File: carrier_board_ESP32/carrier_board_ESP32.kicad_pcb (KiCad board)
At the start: 4 copper layers, 100 x 100 mm, 49 parts, among them J1 Conn_01x02_Socket, J12 LTR390, J13 BME280, J14 ENS160 SPI, J15 ENS160 + AHT21, J16 ENS160 I2C, J17 Conn_01x22_Socket, J18 Conn_01x22_Socket, J2 Conn_01x02_Socket, J3 UJC-HP-3-SMT-TR, U1 TP4056, U2 LM2576HVS-5, U3 MT3608, U4 ESP32-S3-DEVKITC-1-N8R2

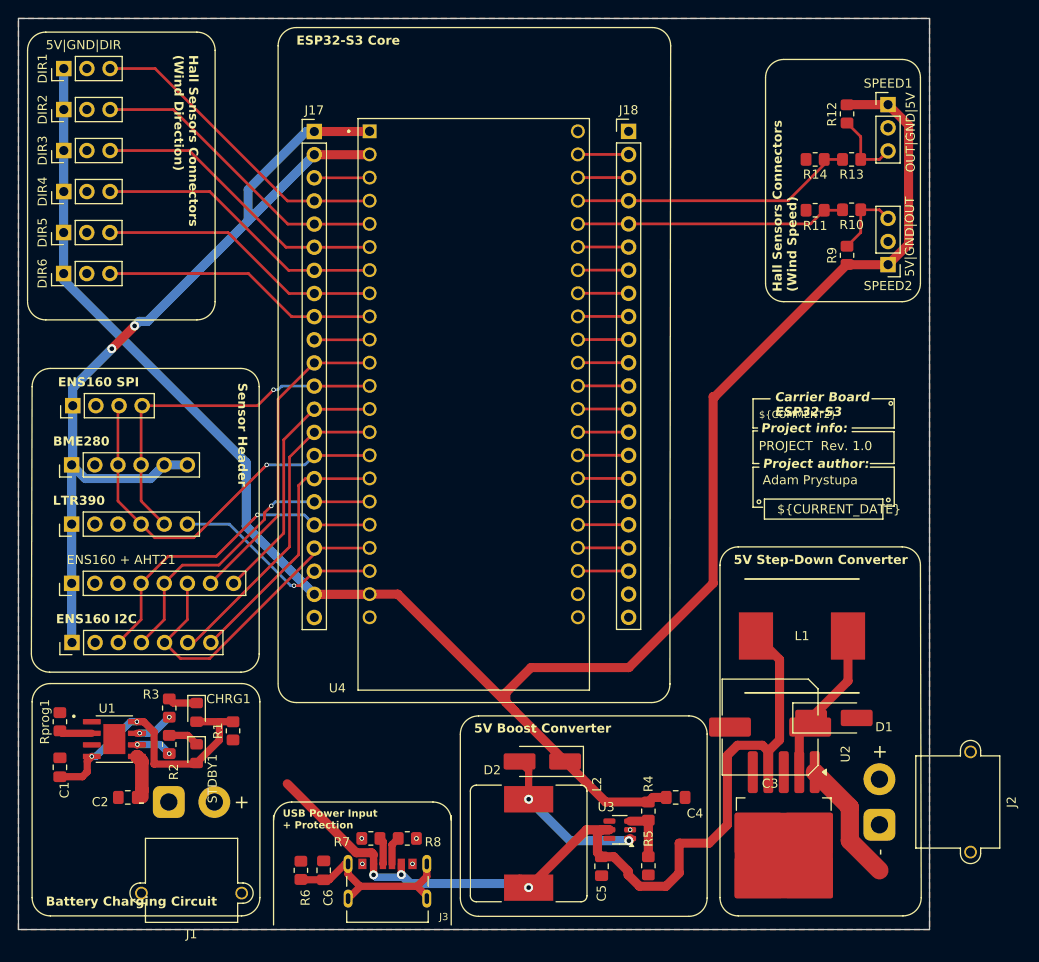
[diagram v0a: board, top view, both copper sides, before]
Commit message: updated scheme and PCB ready for inspection
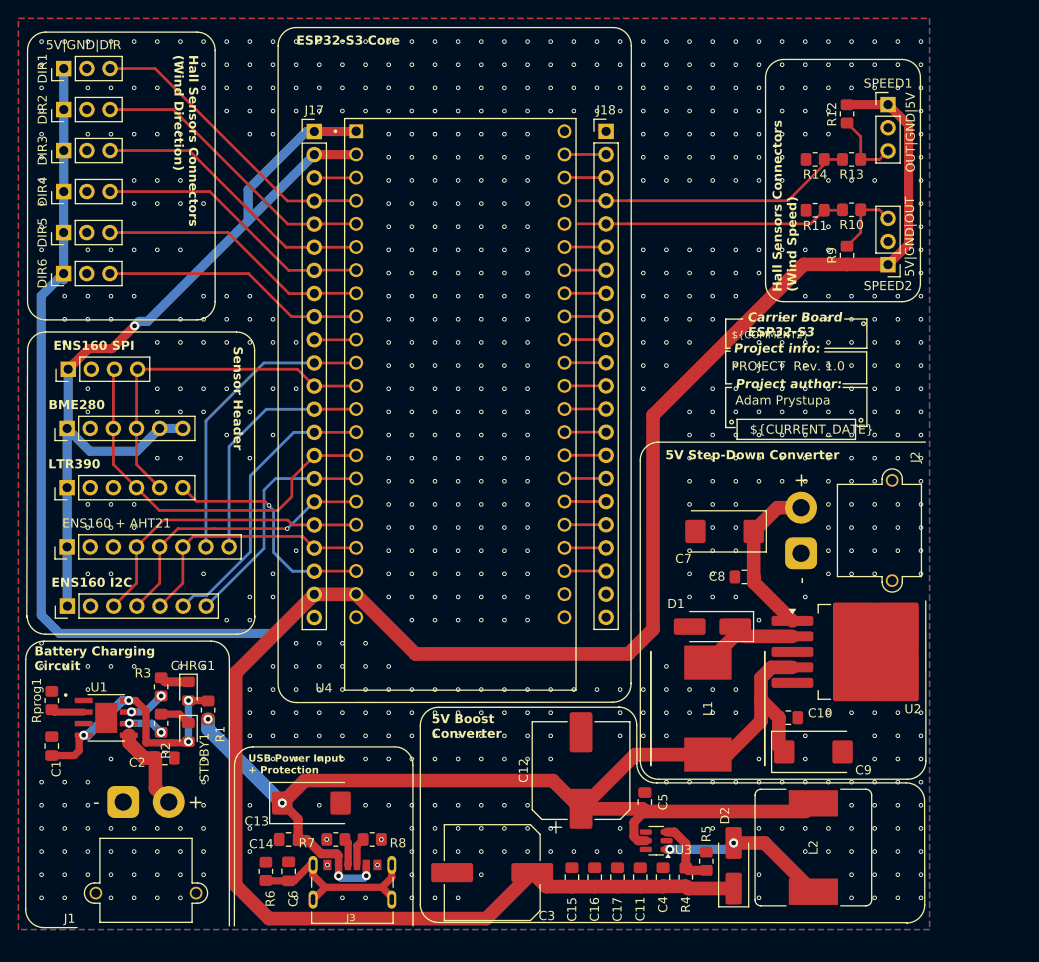
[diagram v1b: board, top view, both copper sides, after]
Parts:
- added C10: 10uF, Capacitor_SMD:C_0805_2012Metric_Pad1.18x1.45mm_HandSolder, F.Cu at (263.0, 98.2)
- added C11: 47uF, Capacitor_SMD:C_0805_2012Metric_Pad1.18x1.45mm_HandSolder, F.Cu at (246.8, 115.8)
- added C12: 2200uF, Capacitor_SMD:CP_Elec_10x10.5, F.Cu at (240.2, 104.0)
- added C13: 10uF, Capacitor_Tantalum_SMD:CP_EIA-7343-15_Kemet-W_Pad2.25x2.55mm_HandSolder, F.Cu at (210.7, 107.6)
- added C14: 1uF, Capacitor_SMD:C_0805_2012Metric_Pad1.18x1.45mm_HandSolder, F.Cu at (208.2, 111.6)
- added C15: 10uF, Capacitor_SMD:C_0805_2012Metric_Pad1.18x1.45mm_HandSolder, F.Cu at (239.2, 115.8)
- added C16: 10uF, Capacitor_SMD:C_0805_2012Metric_Pad1.18x1.45mm_HandSolder, F.Cu at (241.8, 115.8)
- added C17: 10uF, Capacitor_SMD:C_0805_2012Metric_Pad1.18x1.45mm_HandSolder, F.Cu at (244.2, 115.8)
- added C7: 100uF, Capacitor_Tantalum_SMD:CP_EIA-7343-15_Kemet-W_Pad2.25x2.55mm_HandSolder, F.Cu at (256.0, 77.8)
- added C8: 10uF, Capacitor_SMD:C_0805_2012Metric_Pad1.18x1.45mm_HandSolder, F.Cu at (258.2, 82.8)
- added C9: 100uF, Capacitor_Tantalum_SMD:CP_EIA-7343-15_Kemet-W_Pad2.25x2.55mm_HandSolder, F.Cu at (265.8, 102.0)
- moved C3 34.4 mm to (230.5, 115.2)
- moved L2 31.3 mm to (265.8, 112.5), turned to -90 degrees
- moved J2 31.0 mm to (264.4, 80.2)
- moved D2 23.9 mm to (257.0, 114.5), turned to 90 degrees
- moved U2 22.6 mm to (271.1, 91.0), turned to 0 degrees
- moved D1 16.7 mm to (254.7, 88.2), turned to 180 degrees
- moved L1 13.0 mm to (254.2, 97.2), turned to -90 degrees
- moved C4 8.86 mm to (249.2, 115.8), turned to 90 degrees
- moved C5 8.50 mm to (247.2, 107.5), turned to 90 degrees
- moved R4 8.34 mm to (251.8, 115.8), turned to 90 degrees
- moved R5 6.38 mm to (254.0, 114.0), turned to 90 degrees
- moved C2 5.94 mm to (194.6, 102.7)
- moved J1 5.00 mm to (190.0, 107.5)
- moved U3 4.18 mm to (248.5, 111.8)
- moved J12 4.03 mm to (183.8, 73.0)
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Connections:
- C3 pad 1: /5V_supply -> /5V
- J18 pad 17: /GPIO47 -> /5V
- J18 pad 18: /GPIO21 -> /5V
- J18 pad 19: /GPIO20 -> /5V
- J18 pad 20: /GPIO19 -> /5V
- J18 pad 21: GND -> /5V
- J18 pad 22: GND -> /5V
- U4 pad J3_17: /GPIO47 -> /5V
- U4 pad J3_18: /GPIO21 -> /5V
- U4 pad J3_19: /GPIO20 -> /5V
- U4 pad J3_20: /GPIO19 -> /5V
- U4 pad J3_22: GND -> /5V
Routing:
- net /5V: track 217.2 -> 328.3 mm
- net /5V_supply: track 100.4 -> 134.4 mm, vias 3 -> 4
- net /MISO: track 36.2 -> 28.2 mm
- net /GPIO21: track 5.57 -> 0.00 mm
- net /GPIO20: track 5.57 -> 0.00 mm
- net /GPIO19: track 5.57 -> 0.00 mm
- net /GPIO47: track 5.57 -> 0.00 mm
- net Net-(D1-K): track 17.2 -> 11.9 mm
- net /BATT+: track 4.66 -> 9.85 mm
- net /3V3: track 104.6 -> 100.1 mm, vias 2 -> 1
- net /SOLAR+: track 13.7 -> 17.9 mm
- net /INT_3: track 29.3 -> 26.0 mm
- net /SCK: track 36.2 -> 33.1 mm, vias 1 -> 0
- net /MOSI: track 34.2 -> 31.2 mm
- net Net-(CHRG1-A): track 31.8 -> 28.9 mm, vias 2 -> 4
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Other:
- board outline removed
